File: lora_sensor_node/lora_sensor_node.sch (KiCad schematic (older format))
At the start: 1 part

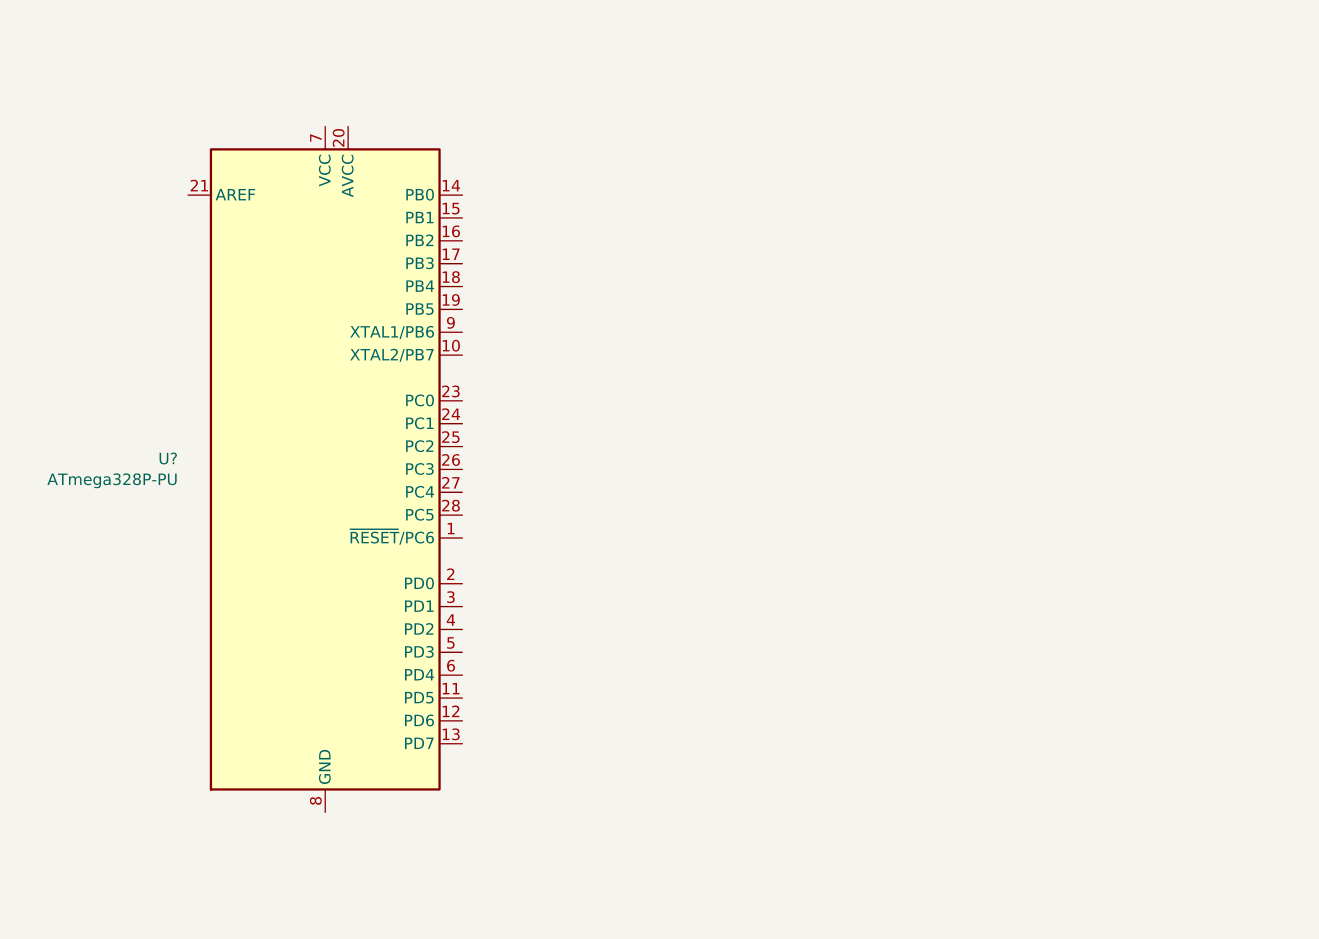
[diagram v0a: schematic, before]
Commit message: Components added
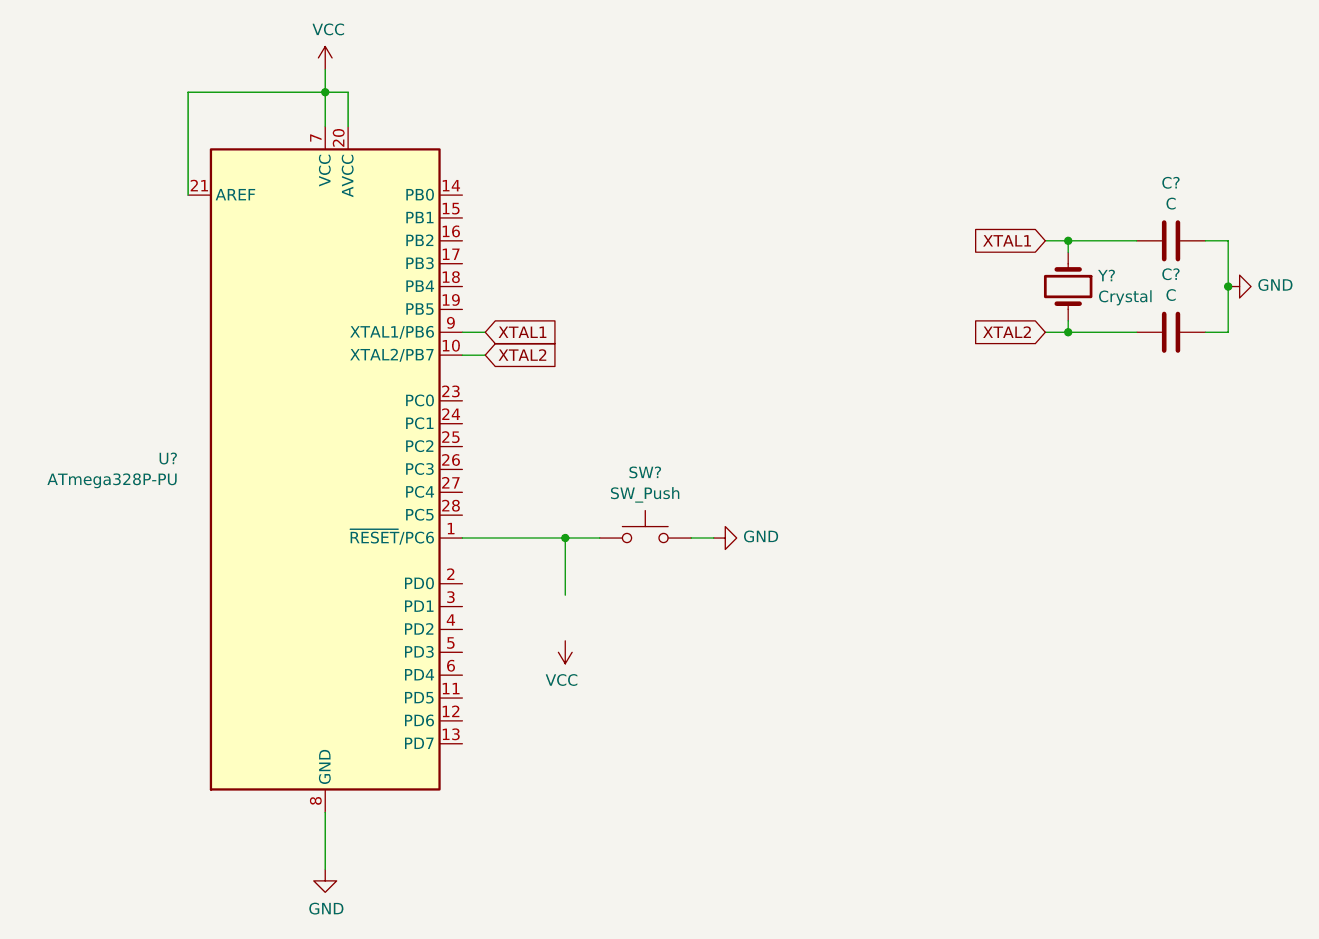
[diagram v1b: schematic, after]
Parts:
- added C? (x2): C, symbol Device:C
- added SW?: SW_Push, symbol Switch:SW_Push
- added Y?: Crystal, symbol Device:Crystal
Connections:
- net labels added: GND, VCC, XTAL1, XTAL2
- wire segments 0 -> 23
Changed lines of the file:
@@
 	1    0    0    -1
 $EndComp
+$Comp
+L power:VCC #PWR?
+U 1 1 5EDB9237
+P 5350 1650
+F 0 "#PWR?" H 5350 1500 50  0001 C CNN
+F 1 "VCC" H 5365 1823 50  0000 C CNN
+F 2 "" H 5350 1650 50  0001 C CNN
+F 3 "" H 5350 1650 50  0001 C CNN
+	1    5350 1650
+	1    0    0    -1
+$EndComp
+$Comp
+L power:GND #PWR?
+U 1 1 5EDB95A0
+P 5350 5150
+F 0 "#PWR?" H 5350 4900 50  0001 C CNN
+F 1 "GND" H 5355 4977 50  0000 C CNN
+F 2 "" H 5350 5150 50  0001 C CNN
+F 3 "" H 5350 5150 50  0001 C CNN
+	1    5350 5150
+	1    0    0    -1
+$EndComp
+Wire Wire Line
+	5350 1900 5350 1750
+Wire Wire Line
+	5450 1900 5450 1750
+Wire Wire Line
+	5450 1750 5350 1750
+Connection ~ 5350 1750
+Wire Wire Line
+	5350 1750 5350 1650
+Wire Wire Line
+	4750 1750 5350 1750
+Wire Wire Line
+	4750 1750 4750 2200
+Wire Wire Line
+	5350 4900 5350 5150
+$Comp
+L Switch:SW_Push SW?
+U 1 1 5EDBAF29
+P 6750 3700
+F 0 "SW?" H 6750 3985 50  0000 C CNN
+F 1 "SW_Push" H 6750 3894 50  0000 C CNN
+F 2 "" H 6750 3900 50  0001 C CNN
+F 3 "~" H 6750 3900 50  0001 C CNN
+	1    6750 3700
+	1    0    0    -1
+$EndComp
+$Comp
+L power:GND #PWR?
+U 1 1 5EDBDCFF
+P 7050 3700
+F 0 "#PWR?" H 7050 3450 50  0001 C CNN
+F 1 "GND" V 7055 3572 50  0000 R CNN
+F 2 "" H 7050 3700 50  0001 C CNN
+F 3 "" H 7050 3700 50  0001 C CNN
+	1    7050 3700
+	0    -1   -1   0
+$EndComp
+Wire Wire Line
+	6950 3700 7050 3700
+$Comp
+L power:VCC #PWR?
+U 1 1 5EDBFA3F
+P 6400 4150
+F 0 "#PWR?" H 6400 4000 50  0001 C CNN
+F 1 "VCC" H 6415 4323 50  0000 C CNN
+F 2 "" H 6400 4150 50  0001 C CNN
+F 3 "" H 6400 4150 50  0001 C CNN
+	1    6400 4150
+	-1   0    0    1
+$EndComp
+Wire Wire Line
+	6400 3950 6400 3700
+Wire Wire Line
+	5950 3700 6400 3700
+Connection ~ 6400 3700
+Wire Wire Line
+	6400 3700 6550 3700
+$Comp
+L Device:C C?
+U 1 1 5EDC7967
+P 9050 2400
+F 0 "C?" V 8798 2400 50  0000 C CNN
+F 1 "C" V 8889 2400 50  0000 C CNN
+F 2 "" H 9088 2250 50  0001 C CNN
+F 3 "~" H 9050 2400 50  0001 C CNN
+	1    9050 2400
+	0    1    1    0
+$EndComp
+$Comp
+L Device:C C?
+U 1 1 5EDC9A3E
+P 9050 2800
+F 0 "C?" V 8798 2800 50  0000 C CNN
+F 1 "C" V 8889 2800 50  0000 C CNN
+F 2 "" H 9088 2650 50  0001 C CNN
+F 3 "~" H 9050 2800 50  0001 C CNN
+	1    9050 2800
+	0    1    1    0
+$EndComp
+$Comp
+L Device:Crystal Y?
+U 1 1 5EDCCC70
+P 8600 2600
+F 0 "Y?" V 8554 2731 50  0000 L CNN
+F 1 "Crystal" V 8645 2731 50  0000 L CNN
+F 2 "" H 8600 2600 50  0001 C CNN
+F 3 "~" H 8600 2600 50  0001 C CNN
+	1    8600 2600
+	0    1    1    0
+$EndComp
+Wire Wire Line
+	8900 2400 8600 2400
+Wire Wire Line
+	8600 2400 8600 2450
+Wire Wire Line
+	8900 2800 8600 2800
+Wire Wire Line
+	8600 2800 8600 2750
+$Comp
+L power:GND #PWR?
+U 1 1 5EDD73FB
+P 9300 2600
+F 0 "#PWR?" H 9300 2350 50  0001 C CNN
+F 1 "GND" V 9305 2472 50  0000 R CNN
+F 2 "" H 9300 2600 50  0001 C CNN
+F 3 "" H 9300 2600 50  0001 C CNN
+	1    9300 2600
+	0    -1   -1   0
+$EndComp
+Wire Wire Line
+	9200 2400 9300 2400
+Wire Wire Line
+	9300 2400 9300 2600
+Wire Wire Line
+	9200 2800 9300 2800
+Wire Wire Line
+	9300 2800 9300 2600
+Connection ~ 9300 2600
+Text GLabel 6050 2800 2    50   Input ~ 0
+XTAL1
+Text GLabel 8500 2400 0    50   Input ~ 0
+XTAL1
+Text GLabel 6050 2900 2    50   Input ~ 0
+XTAL2
+Text GLabel 8500 2800 0    50   Input ~ 0
+XTAL2
+Wire Wire Line
+	5950 2800 6050 2800
+Wire Wire Line
+	5950 2900 6050 2900
+Wire Wire Line
+	8600 2400 8500 2400
+Connection ~ 8600 2400
+Wire Wire Line
+	8600 2800 8500 2800
+Connection ~ 8600 2800
 $EndSCHEMATC
